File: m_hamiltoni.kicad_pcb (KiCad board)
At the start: 2 copper layers, 39 parts, among them J1 MJ-4PP-9, J3 OLED, U1 ProMicro_r

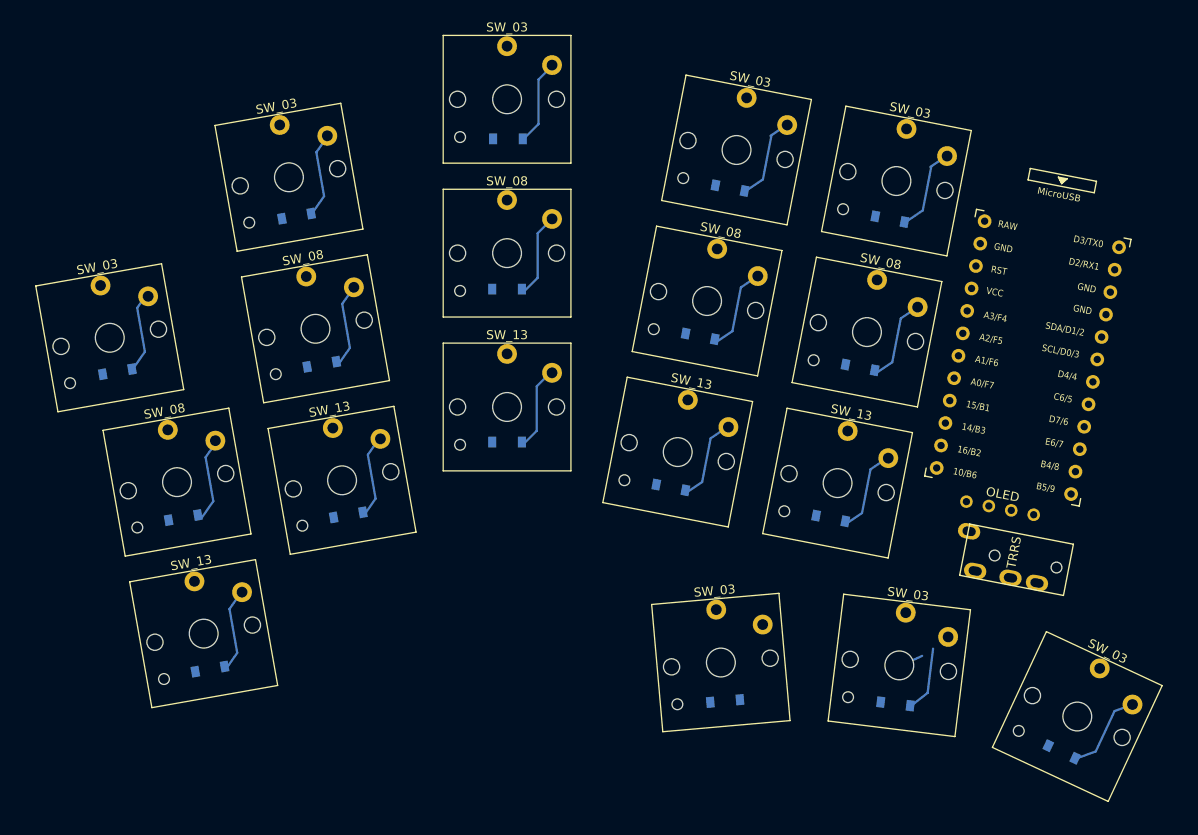
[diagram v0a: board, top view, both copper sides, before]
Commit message: Draft an outline for the PCB
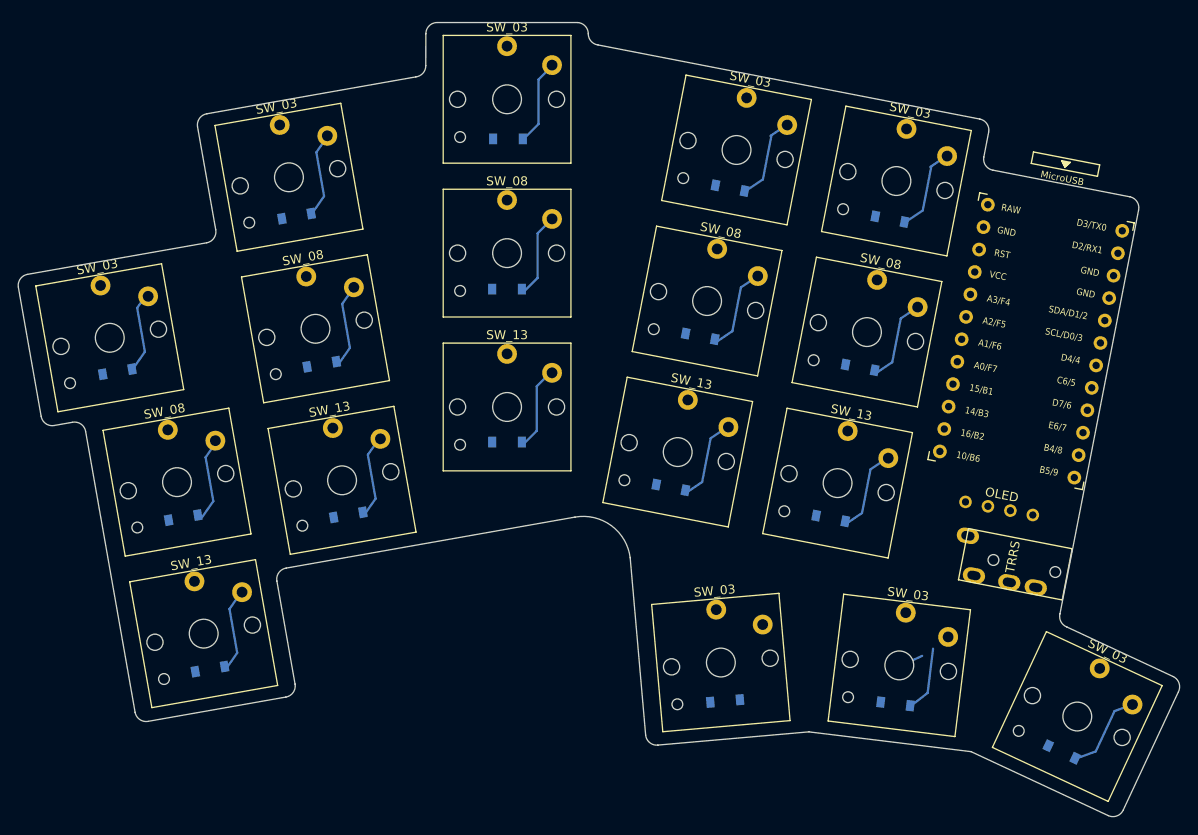
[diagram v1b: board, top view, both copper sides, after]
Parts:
- moved U1 1.87 mm to (-28.9, 10.3)
- moved J1 0.52 mm to (-24.6, 35.7)
- moved J3 0.10 mm to (-32.3, 28.4)
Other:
- board outline added: 129.1 x 88.3 mm
